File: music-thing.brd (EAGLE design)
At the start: 55.9 x 61 mm, 6 parts

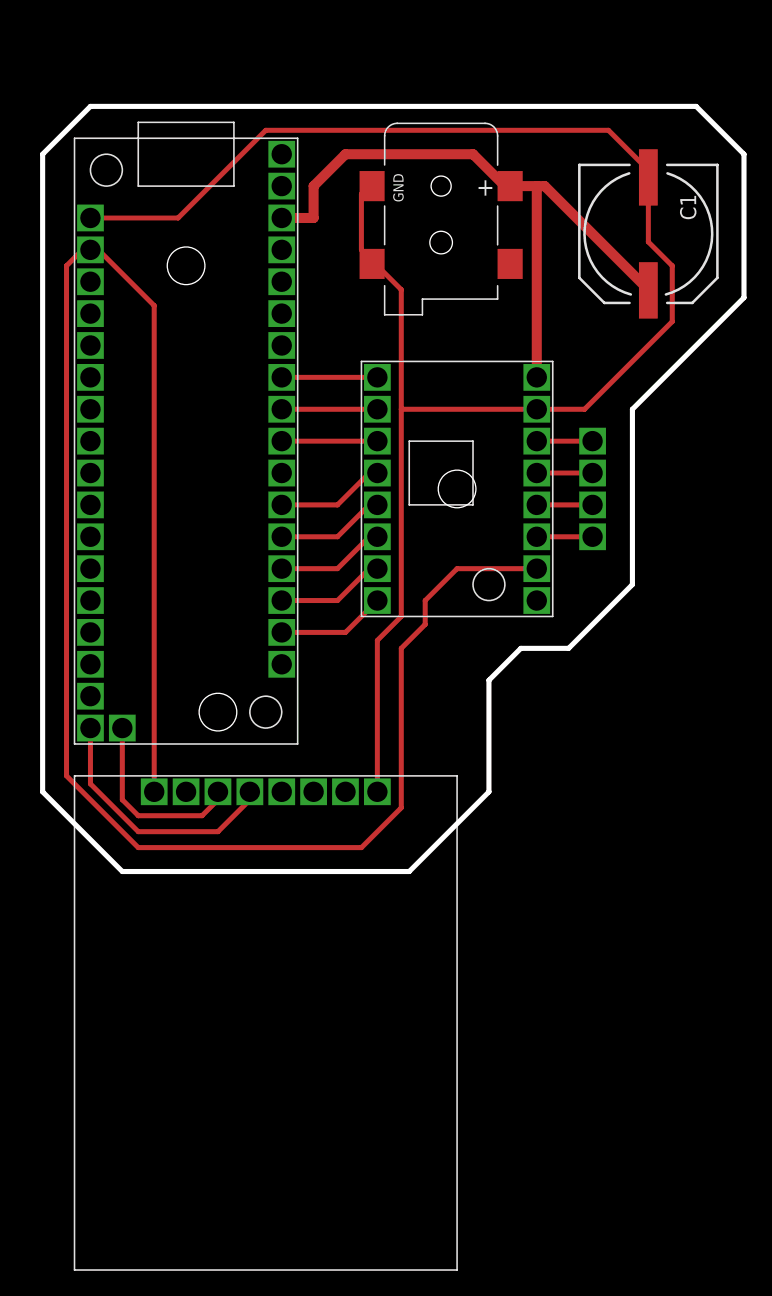
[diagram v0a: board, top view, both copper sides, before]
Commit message: new layout
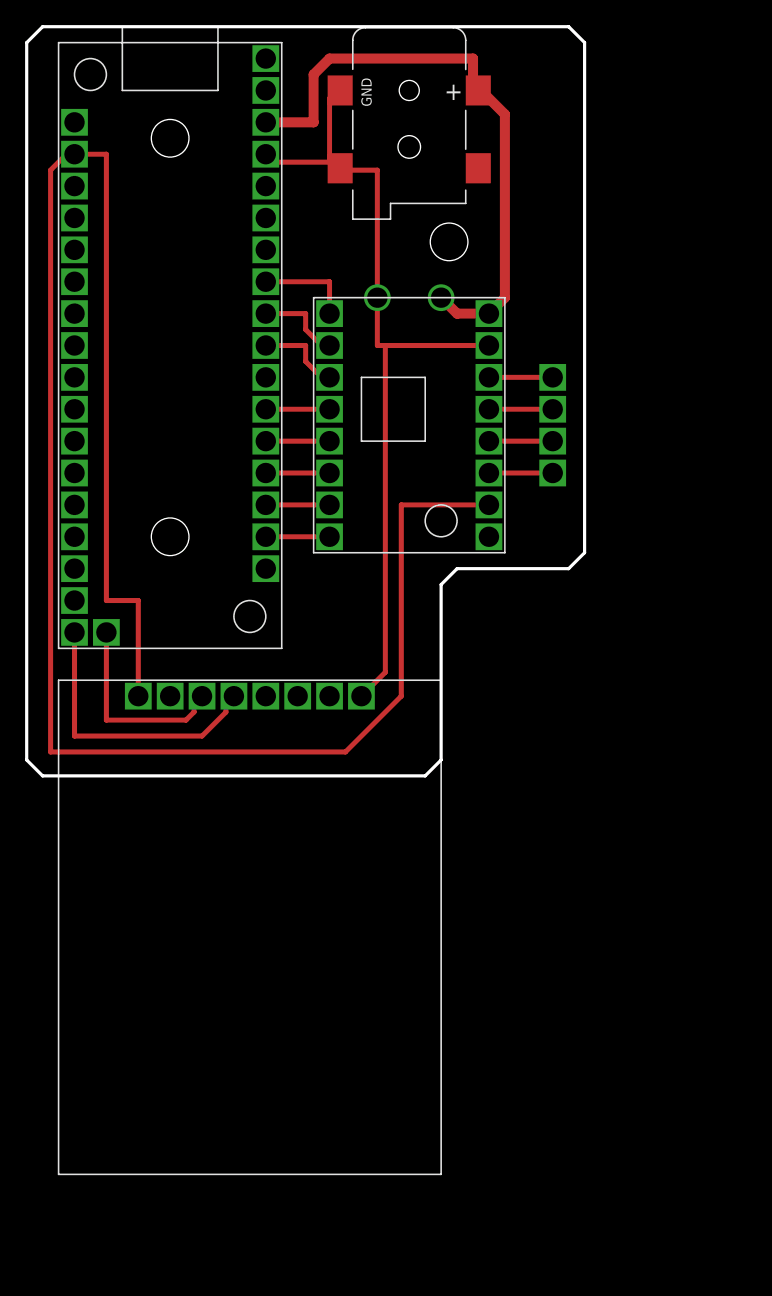
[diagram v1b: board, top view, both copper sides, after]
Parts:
- removed C1: 100uF, SparkFun-Capacitors:NIC_10X10.5_CAP
- moved CN1 8.03 mm to (30.5, 74.9)
- moved U$2 7.73 mm to (2.54, 30.5)
- moved U$3 7.73 mm to (33.0, -11.4)
- moved U$1 6.35 mm to (22.9, 38.1)
- moved U$4 5.99 mm to (39.4, 44.5)
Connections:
- removed net N$5: C1.+, CN1.PWR1, U$1.VMOT, U$2.VIN
- new net N$16: CN1.PWR1, U$1.VMOT, U$2.VIN
- net GND: now also U$2.GND2; no longer C1.-, U$2.GND1
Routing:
- net GND: track 136.9 -> 68.6 mm, vias 0 -> 1
- net N$5: track 52.6 -> 0.00 mm
- net N$16: track 0.00 -> 47.5 mm, vias 0 -> 1
- net N$10: track 8.67 -> 5.08 mm
- net N$9: track 8.67 -> 5.08 mm
- net N$8: track 8.67 -> 5.08 mm
- net N$7: track 8.67 -> 5.08 mm
- net N$6: track 8.67 -> 5.08 mm
- net 5V: track 146.3 -> 149.1 mm
- net N$15: track 20.4 -> 22.6 mm
- net N$12: track 7.62 -> 6.88 mm
- net N$11: track 7.62 -> 6.88 mm
- net N$14: track 15.0 -> 15.8 mm
- net N$4: track 4.45 -> 5.08 mm
- net N$3: track 4.45 -> 5.08 mm
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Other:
- board size 55.9 x 61 mm -> 44.5 x 59.7 mm
